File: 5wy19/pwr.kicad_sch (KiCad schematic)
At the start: 16 parts, among them IC7 A2C20219

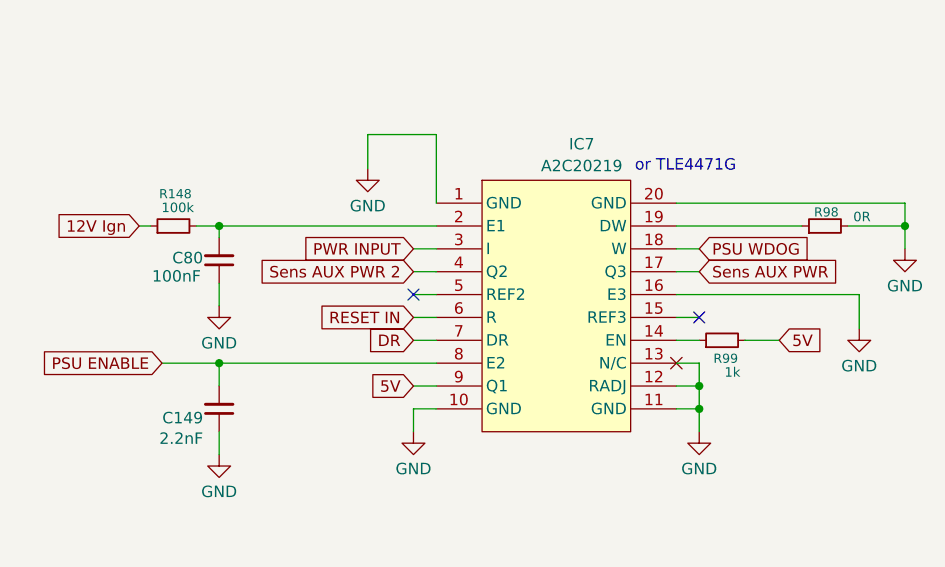
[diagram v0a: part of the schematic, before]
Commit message: Final schematic (except maybe some oversights)
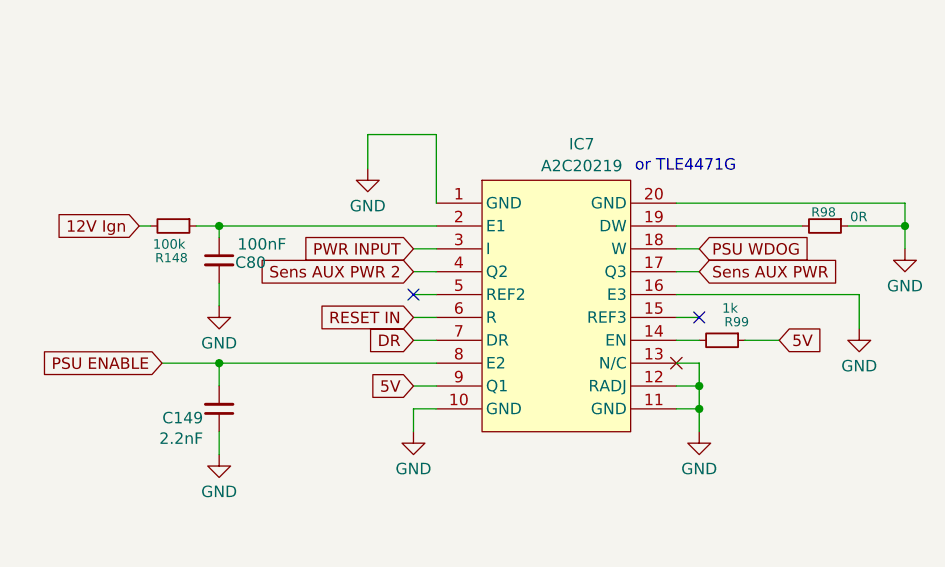
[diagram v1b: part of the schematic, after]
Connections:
- net 12V Ign: now also R148.2; no longer R148.1
- net 5V: now also R99.1; no longer R99.2
- net GND: now also C80.2, R98.1; no longer C80.1, R98.2
- net at IC7.14 (EN): now also R99.2; no longer R99.1
- net at IC7.19 (DW): now also R98.2; no longer R98.1
- new net: C80.1, IC7.2 (E1), R148.1
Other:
- moved on the sheet: C80, R148, R98, R99
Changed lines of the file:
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@@
 	(symbol
 		(lib_id "Device:R_Small")
-		(at 101.6 87.63 90)
+		(at 101.6 87.63 270)
 		(unit 1)
 		(exclude_from_sim no)
@@
 		(dnp no)
 		(property "Reference" "R148"
-			(at 103.632 84.074 90)
+			(at 99.568 91.186 90)
 			(effects
 				(font
@@
 		)
 		(property "Value" "100k"
-			(at 103.886 85.598 90)
+			(at 99.314 89.662 90)
 			(effects
 				(font
@@
 	(symbol
 		(lib_id "Device:R_Small")
-		(at 162.56 100.33 90)
+		(at 162.56 100.33 270)
 		(unit 1)
 		(exclude_from_sim no)
@@
 		(dnp no)
 		(property "Reference" "R99"
-			(at 164.338 102.362 90)
+			(at 162.814 98.298 90)
 			(effects
 				(font
@@
 		)
 		(property "Value" "1k"
-			(at 164.592 103.886 90)
+			(at 162.56 96.774 90)
 			(effects
 				(font
@@
 	(symbol
 		(lib_id "Device:C_Small")
-		(at 106.68 91.44 180)
+		(at 106.68 91.44 0)
 		(unit 1)
 		(exclude_from_sim no)
@@
 		(dnp no)
 		(property "Reference" "C80"
-			(at 104.902 91.186 0)
+			(at 108.458 91.694 0)
 			(effects
 				(font
@@
 		)
 		(property "Value" "100nF"
-			(at 104.648 93.218 0)
+			(at 108.712 89.662 0)
 			(effects
 				(font
@@
 	(symbol
 		(lib_id "Device:R_Small")
-		(at 173.99 87.63 90)
+		(at 173.99 87.63 270)
 		(unit 1)
 		(exclude_from_sim no)
@@
 		(dnp no)
 		(property "Reference" "R98"
-			(at 175.514 86.106 90)
+			(at 172.466 86.106 90)
 			(effects
 				(font
@@
 		)
 		(property "Value" "0R"
-			(at 179.07 86.614 90)
-			(effects
-				(font
+			(at 176.784 86.614 90)
+			(effects
+				(font
